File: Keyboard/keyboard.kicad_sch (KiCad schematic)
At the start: 2 parts, among them SW1 SW_Push

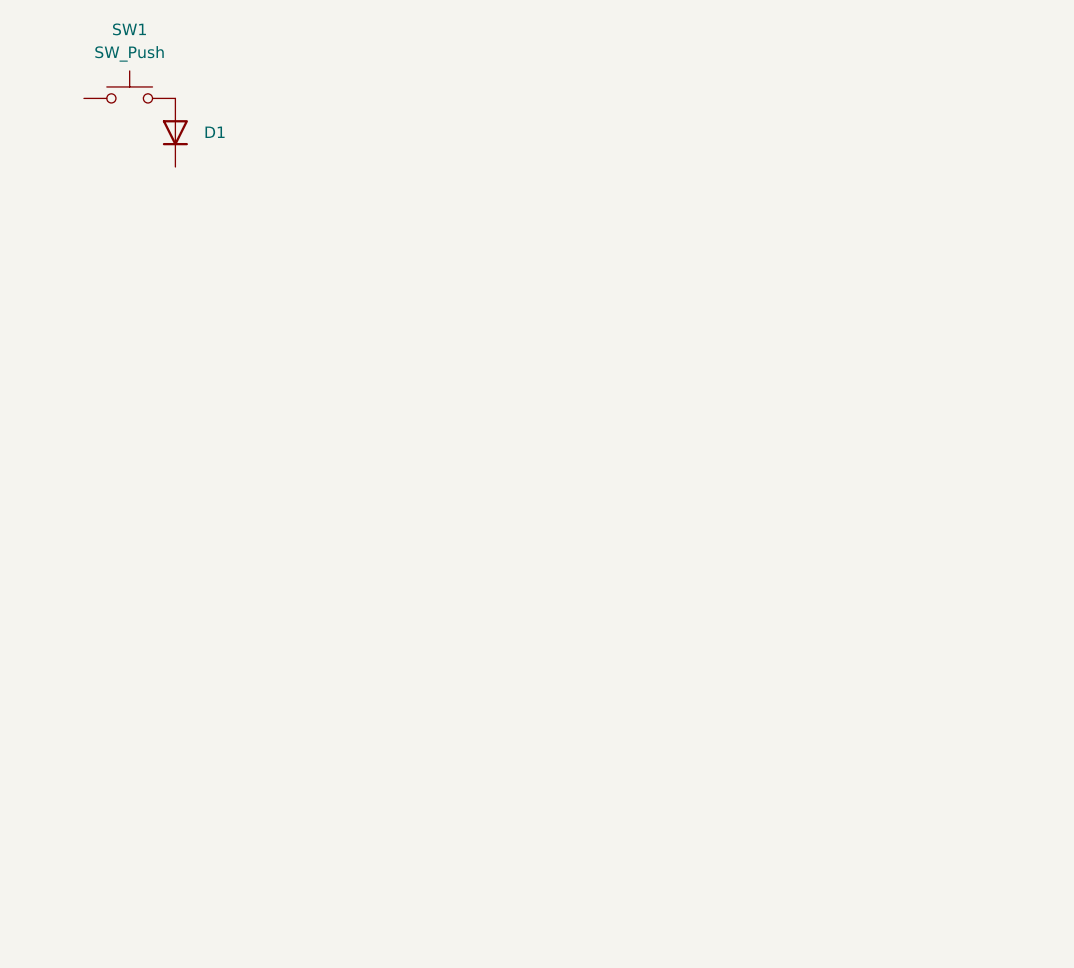
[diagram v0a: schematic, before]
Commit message: Fixed minor issues & plotted gerber
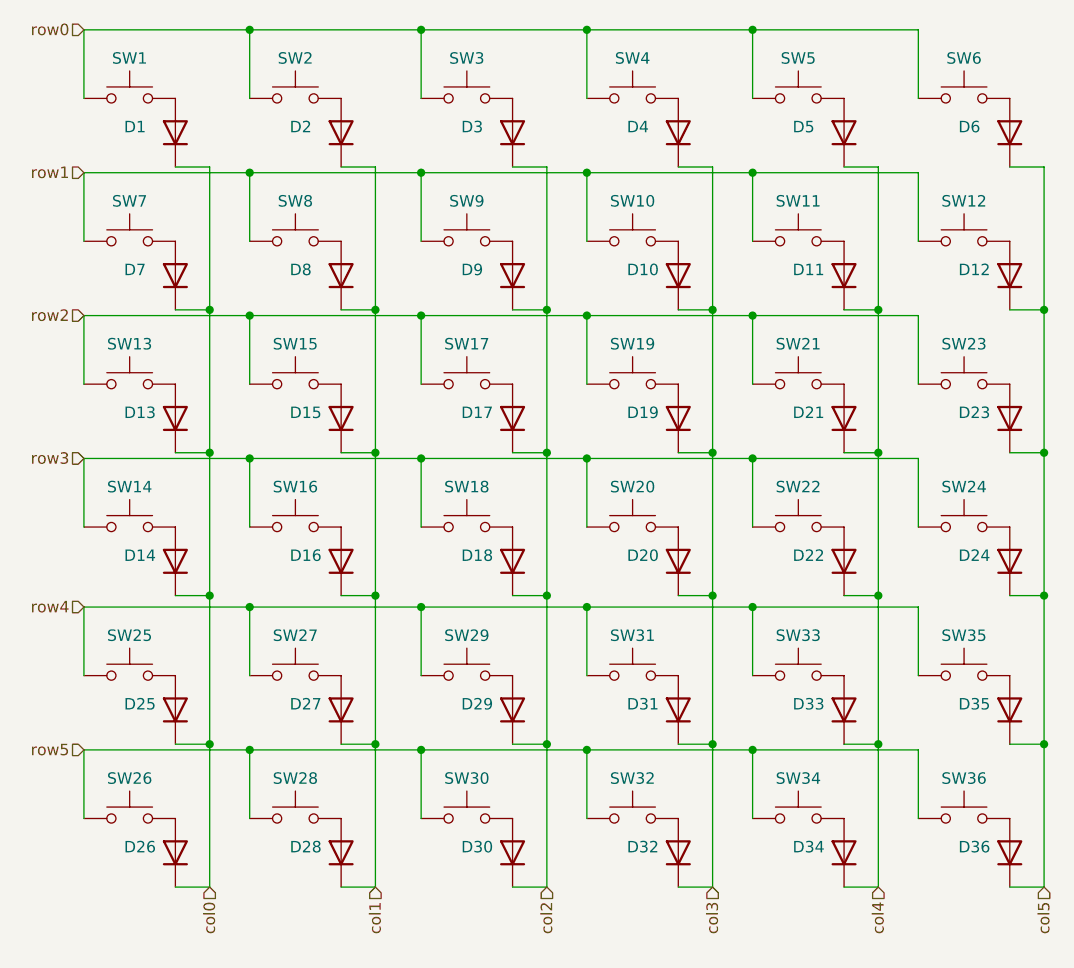
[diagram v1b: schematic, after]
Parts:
- added D10, D11, D12, D13, D14, D15, D16, D17, D18, D19, D2, D20, D21, D22, D23, D24, D25, D26, D27, D28, D29, D3, D30, D31, D32, D33, D34, D35, D36, D4, D5, D6, D7, D8, D9: 1N4148WS, Diode_SMD:D_SOD-323, symbol Diode:1N4148WS
- added SW10, SW11, SW12, SW13, SW14, SW15, SW16, SW17, SW18, SW19, SW2, SW20, SW21, SW22, SW23, SW24, SW25, SW26, SW27, SW28, SW29, SW3, SW30, SW31, SW32, SW33, SW34, SW35, SW36, SW4, SW5, SW6, SW7, SW8, SW9: SW_Push, button:SW_TL3315NF250Q, symbol Switch:SW_Push
- SW1: footprint (none) -> button:SW_TL3315NF250Q
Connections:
- net col0: now reaches D1.1 (K)
- net col0: now also D13.1 (K), D14.1 (K), D25.1 (K), D26.1 (K), D7.1 (K)
- net row0: now reaches SW1.1
- net row0: now also SW2.1, SW3.1, SW4.1, SW5.1, SW6.1
- new net: D24.2 (A), SW24.2
- new net: D16.2 (A), SW16.2
- new net: D32.2 (A), SW32.2
- new net: D11.2 (A), SW11.2
- new net: D34.2 (A), SW34.2
- new net: D7.2 (A), SW7.2
- new net: D19.2 (A), SW19.2
- new net: D15.2 (A), SW15.2
- new net: D6.2 (A), SW6.2
- new net: D14.2 (A), SW14.2
- new net: D31.2 (A), SW31.2
- new net: D20.2 (A), SW20.2
- new net: D18.2 (A), SW18.2
- new net: D30.2 (A), SW30.2
- new net: D10.2 (A), SW10.2
- new net: D36.2 (A), SW36.2
- new net: D29.2 (A), SW29.2
- new net: D8.2 (A), SW8.2
- new net: D4.2 (A), SW4.2
- new net: D3.2 (A), SW3.2
- new net: D28.2 (A), SW28.2
- new net: D35.2 (A), SW35.2
- new net: D5.2 (A), SW5.2
- new net: D33.2 (A), SW33.2
- new net: D22.2 (A), SW22.2
- new net: D25.2 (A), SW25.2
- new net: D12.2 (A), SW12.2
- new net: D13.2 (A), SW13.2
- new net: D26.2 (A), SW26.2
- new net: D2.2 (A), SW2.2
- new net: D27.2 (A), SW27.2
- new net: D23.2 (A), SW23.2
- new net: D21.2 (A), SW21.2
- new net: D17.2 (A), SW17.2
- new net: D9.2 (A), SW9.2
- new net col1: D15.1 (K), D16.1 (K), D2.1 (K), D27.1 (K), D28.1 (K), D8.1 (K)
- new net col2: D17.1 (K), D18.1 (K), D29.1 (K), D3.1 (K), D30.1 (K), D9.1 (K)
- new net col3: D10.1 (K), D19.1 (K), D20.1 (K), D31.1 (K), D32.1 (K), D4.1 (K)
- new net col4: D11.1 (K), D21.1 (K), D22.1 (K), D33.1 (K), D34.1 (K), D5.1 (K)
- new net col5: D12.1 (K), D23.1 (K), D24.1 (K), D35.1 (K), D36.1 (K), D6.1 (K)
- new net row1: SW10.1, SW11.1, SW12.1, SW7.1, SW8.1, SW9.1
- new net row2: SW13.1, SW15.1, SW17.1, SW19.1, SW21.1, SW23.1
- new net row3: SW14.1, SW16.1, SW18.1, SW20.1, SW22.1, SW24.1
- new net row4: SW25.1, SW27.1, SW29.1, SW31.1, SW33.1, SW35.1
- new net row5: SW26.1, SW28.1, SW30.1, SW32.1, SW34.1, SW36.1
